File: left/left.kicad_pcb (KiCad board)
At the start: 2 copper layers, 158.5 x 116.8 mm, 57 parts, among them J1 MJ-4PP-9, U1 ProMicro

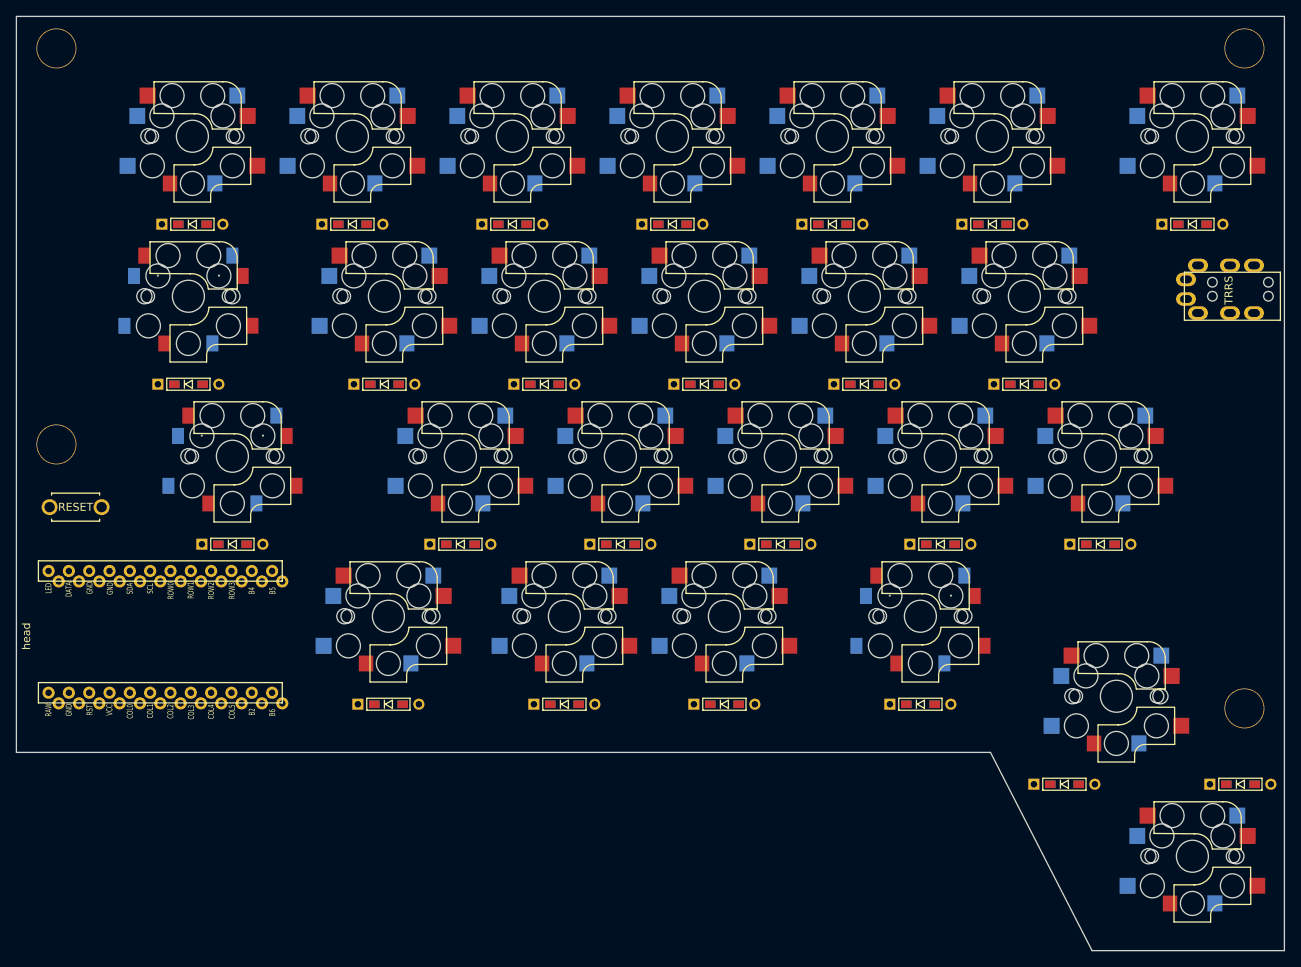
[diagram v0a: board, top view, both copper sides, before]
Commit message: 左手PCB完成
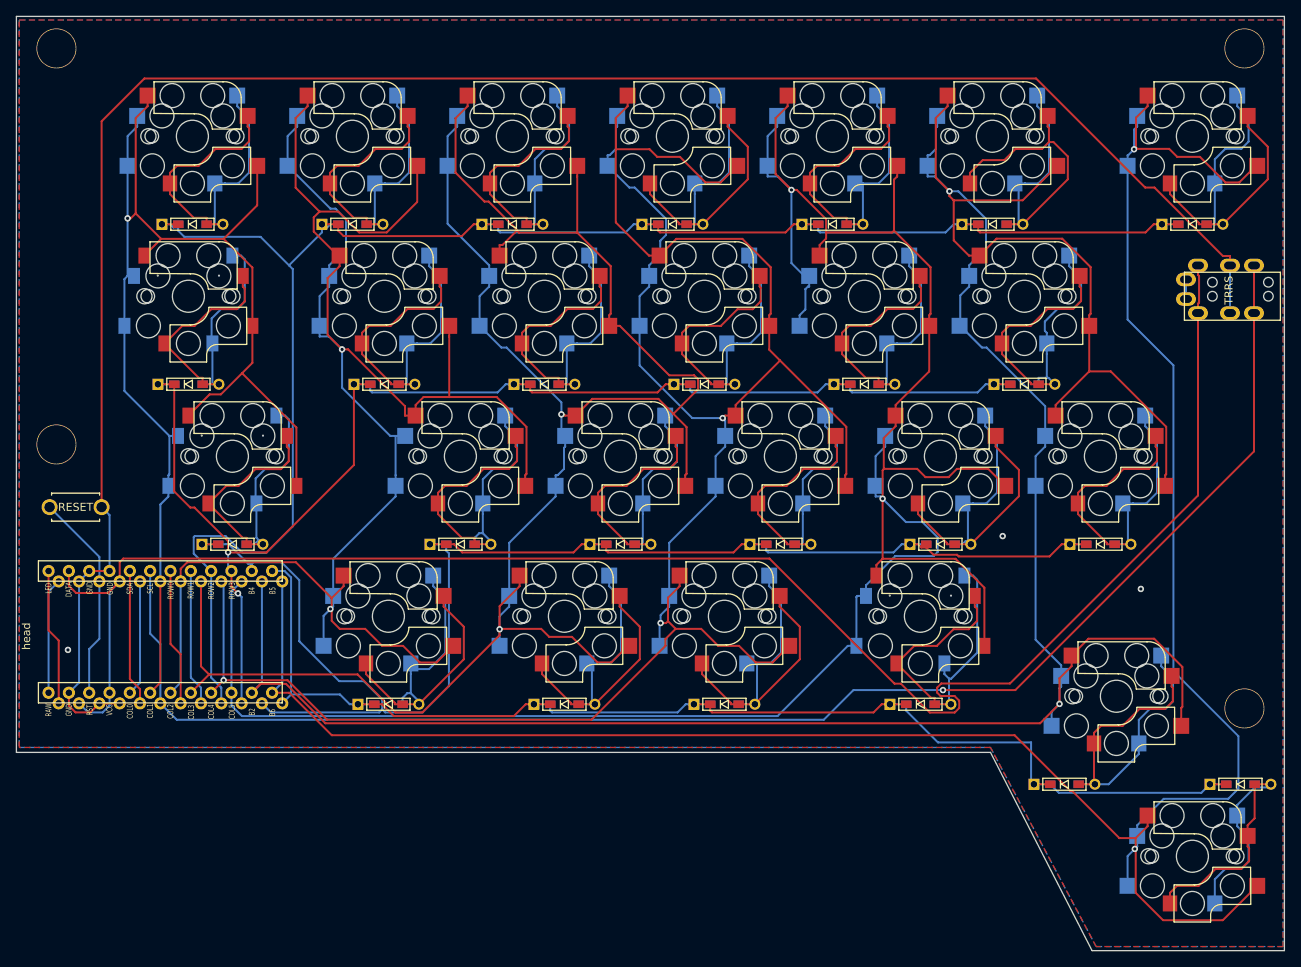
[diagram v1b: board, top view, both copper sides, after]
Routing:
- net col6: track 0.00 -> 333.7 mm, vias 0 -> 2
- net col7: track 0.00 -> 296.9 mm, vias 0 -> 2
- net col5: track 0.00 -> 295.4 mm, vias 0 -> 2
- net col4: track 0.00 -> 285.7 mm, vias 0 -> 3
- net col3: track 0.00 -> 262.3 mm, vias 0 -> 2
- net col2: track 0.00 -> 246.2 mm, vias 0 -> 2
- net GND: track 0.00 -> 243.8 mm, vias 0 -> 3
- net row1: track 0.00 -> 223.7 mm
- net pwr: track 0.00 -> 221.7 mm
- net data: track 0.00 -> 191.8 mm, vias 0 -> 1
- net row3: track 0.00 -> 180.1 mm
- net row2: track 0.00 -> 175.6 mm, vias 0 -> 2
- net col1: track 0.00 -> 165.3 mm, vias 0 -> 1
- net row4: track 0.00 -> 160.7 mm
- net Net-(D6-A): track 0.00 -> 54.3 mm
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- added copper zone on B.Cu, net GND
- added copper zone on F.Cu, net GND
